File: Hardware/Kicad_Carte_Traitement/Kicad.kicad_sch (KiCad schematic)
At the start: 24 parts, among them J1 Conn_02x07_Odd_Even, J5 DA15_Receptacle_MountingHoles, U2 STM32G474RETx

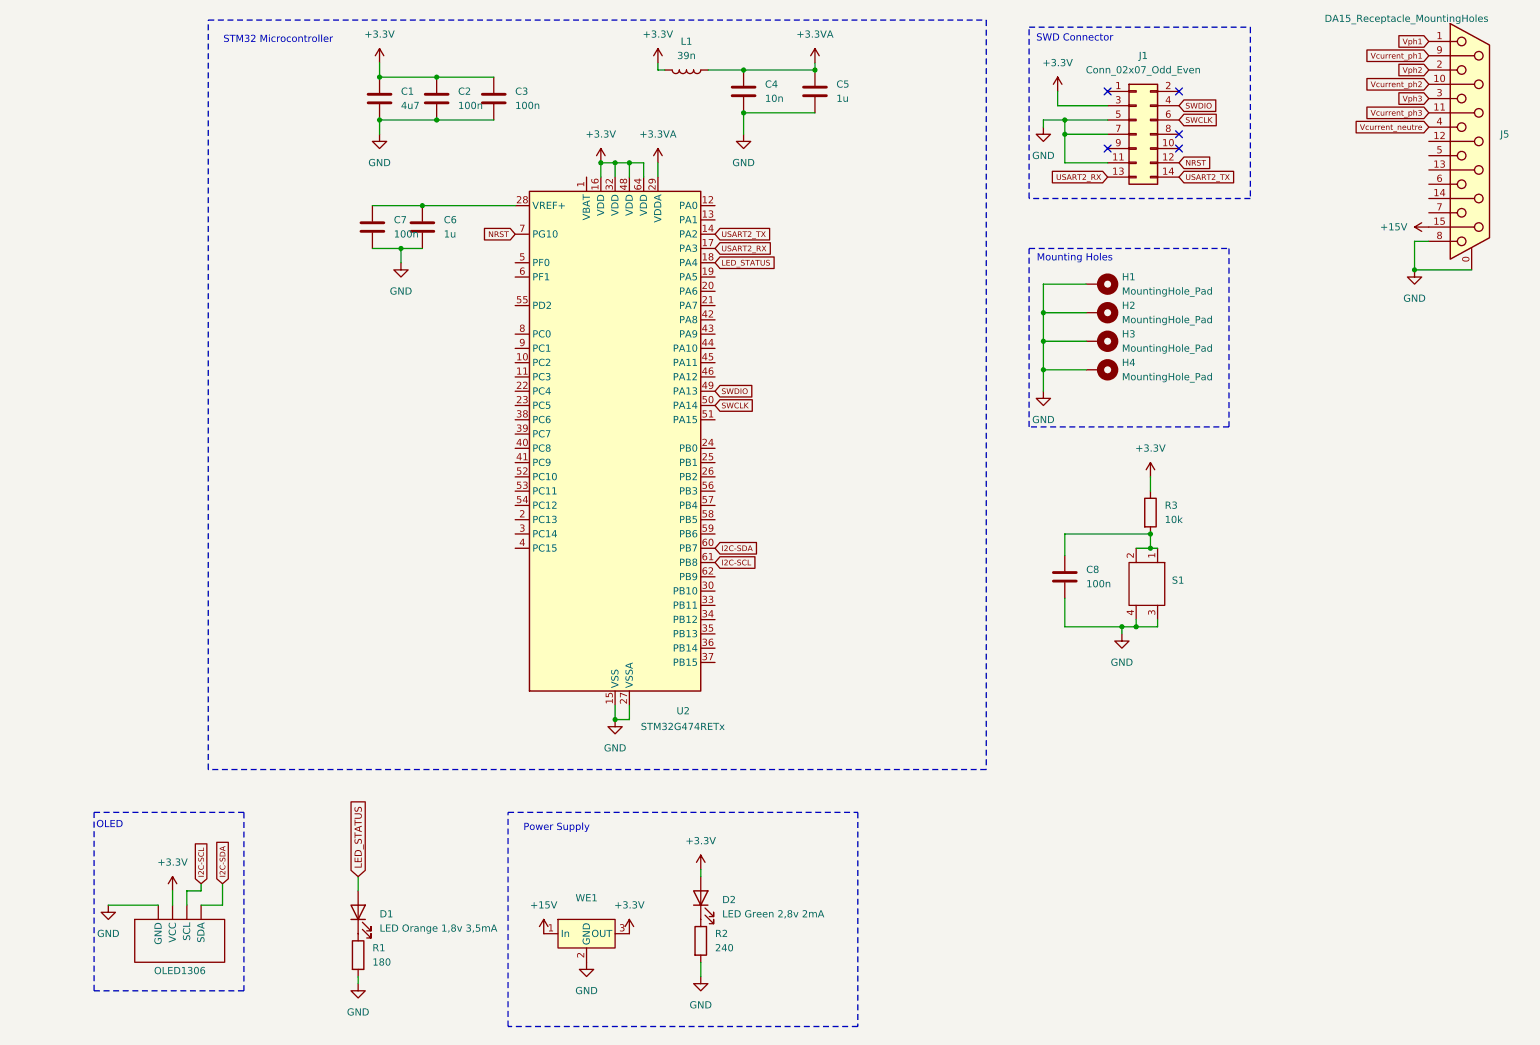
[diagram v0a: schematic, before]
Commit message: MAJ
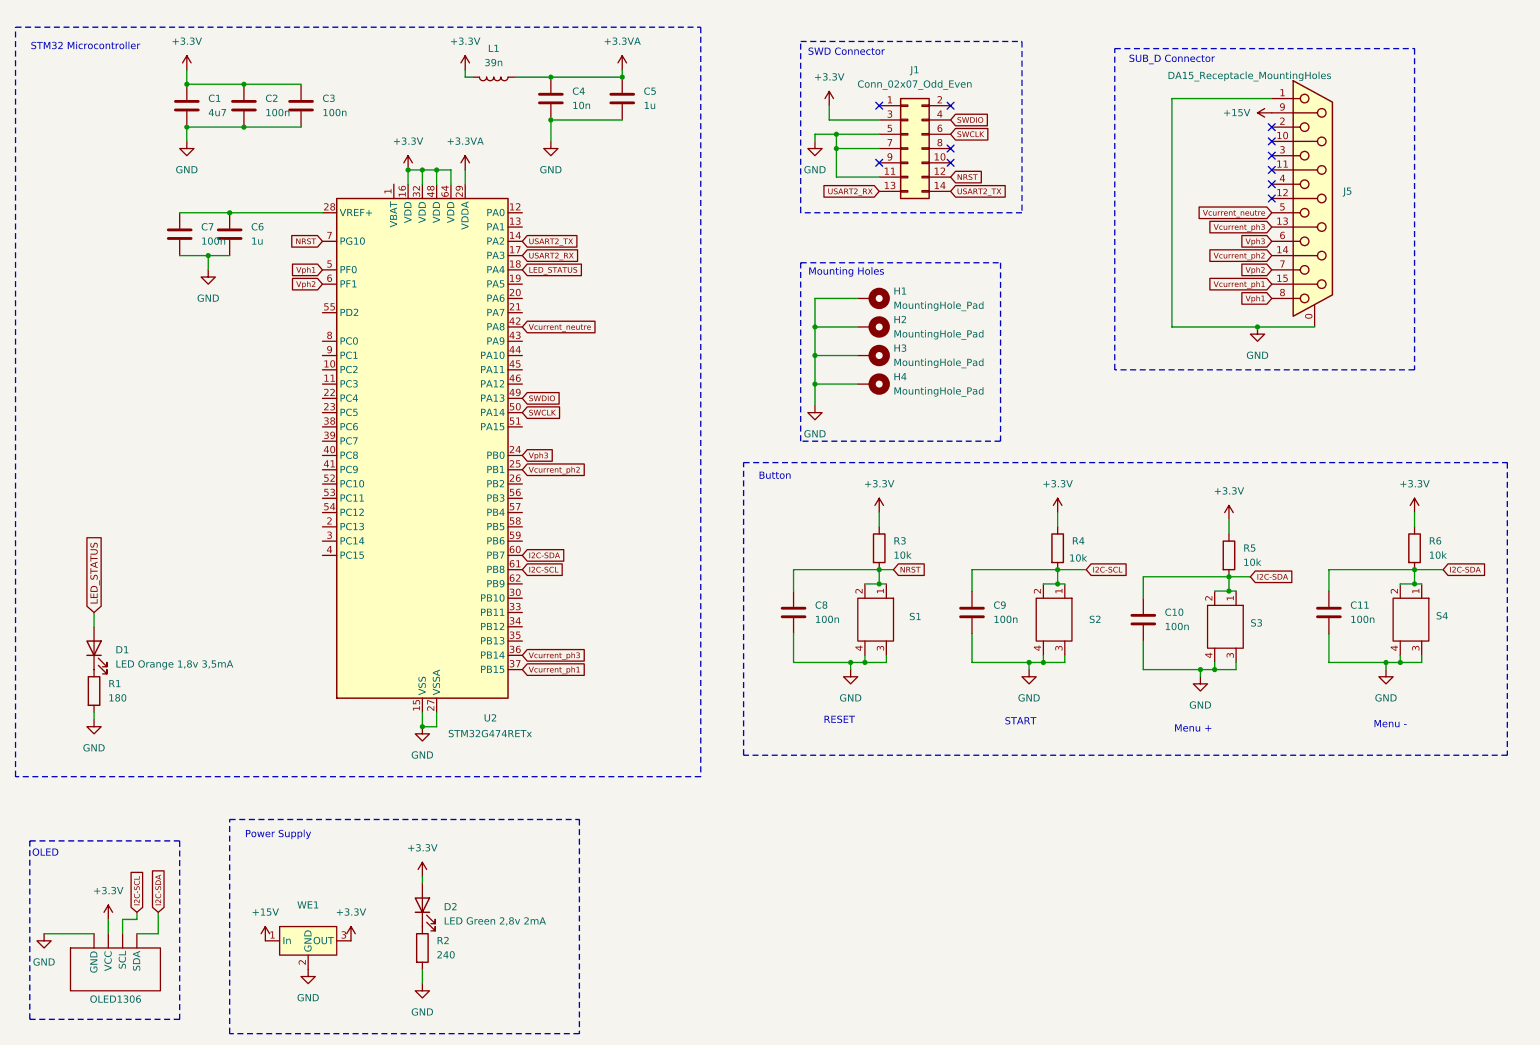
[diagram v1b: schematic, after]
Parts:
- added C10, C11, C9: 100n, symbol Device:C
- added R4, R5, R6: 10k, symbol Device:R
- added S2, S3, S4: ~, Switch:Tact_switch, symbol switch:Tact_switch
- J5: footprint (none) -> Library.pretty_SUBD:SUB_D
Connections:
- net +15V: now also J5.9 (P9); no longer J5.15 (P15)
- net +3.3V: now also R4.1, R5.1, R6.1
- net GND: now also J5.1, C10.2, C11.2, C9.2, S2.3, S2.4, S3.3, S3.4, S4.3, S4.4; no longer J5.8
- net I2C-SCL: now also C9.1, R4.2, S2.1, S2.2
- net I2C-SDA: now also C10.1, C11.1, R5.2, R6.2, S3.1, S3.2, S4.1, S4.2
- net NRST: now also C8.1, R3.2, S1.1, S1.2
- net Vcurrent_neutre: now also J5.5, U2.42 (PA8); no longer J5.4
- net Vcurrent_ph1: now also J5.15 (P15), U2.37 (PB15); no longer J5.9 (P9)
- net Vcurrent_ph2: now also J5.14 (P14), U2.25 (PB1); no longer J5.10 (P10)
- net Vcurrent_ph3: now also J5.13 (P13), U2.36 (PB14); no longer J5.11 (P111)
- net Vph1: now also J5.8, U2.5 (PF0); no longer J5.1
- net Vph2: now also J5.7, U2.6 (PF1); no longer J5.2
- net Vph3: now also J5.6, U2.24 (PB0); no longer J5.3
- no-connect marks 5 -> 11
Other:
- note added: "Button"
- note added: "Menu +"
- note added: "Menu -"
- note added: "RESET"
- note added: "START"
- note added: "SUB_D Connector"
- moved on the sheet: C1, C2, C3, C4, C5, C6, C7, C8, D1, D2, H1, H2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
